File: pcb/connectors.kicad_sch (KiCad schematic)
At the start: 5 parts, among them CN1 STDC14, CN2 SM04B-SRSS-TB (LF)(SN), CN4 SM04B-SRSS-TB (LF)(SN), J1 Conn_01x12, J2 Conn_01x16

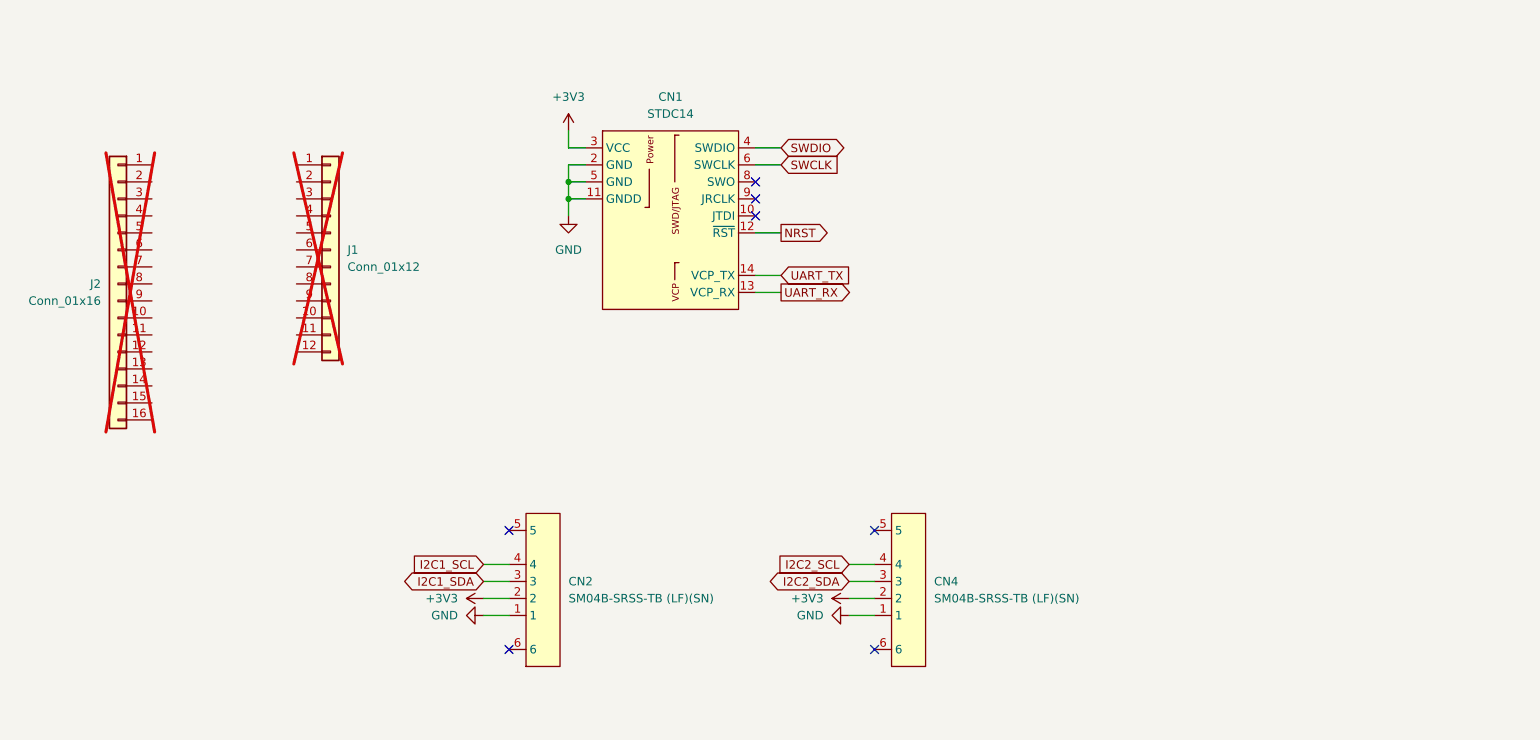
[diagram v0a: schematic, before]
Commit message: Lots of work on schematics
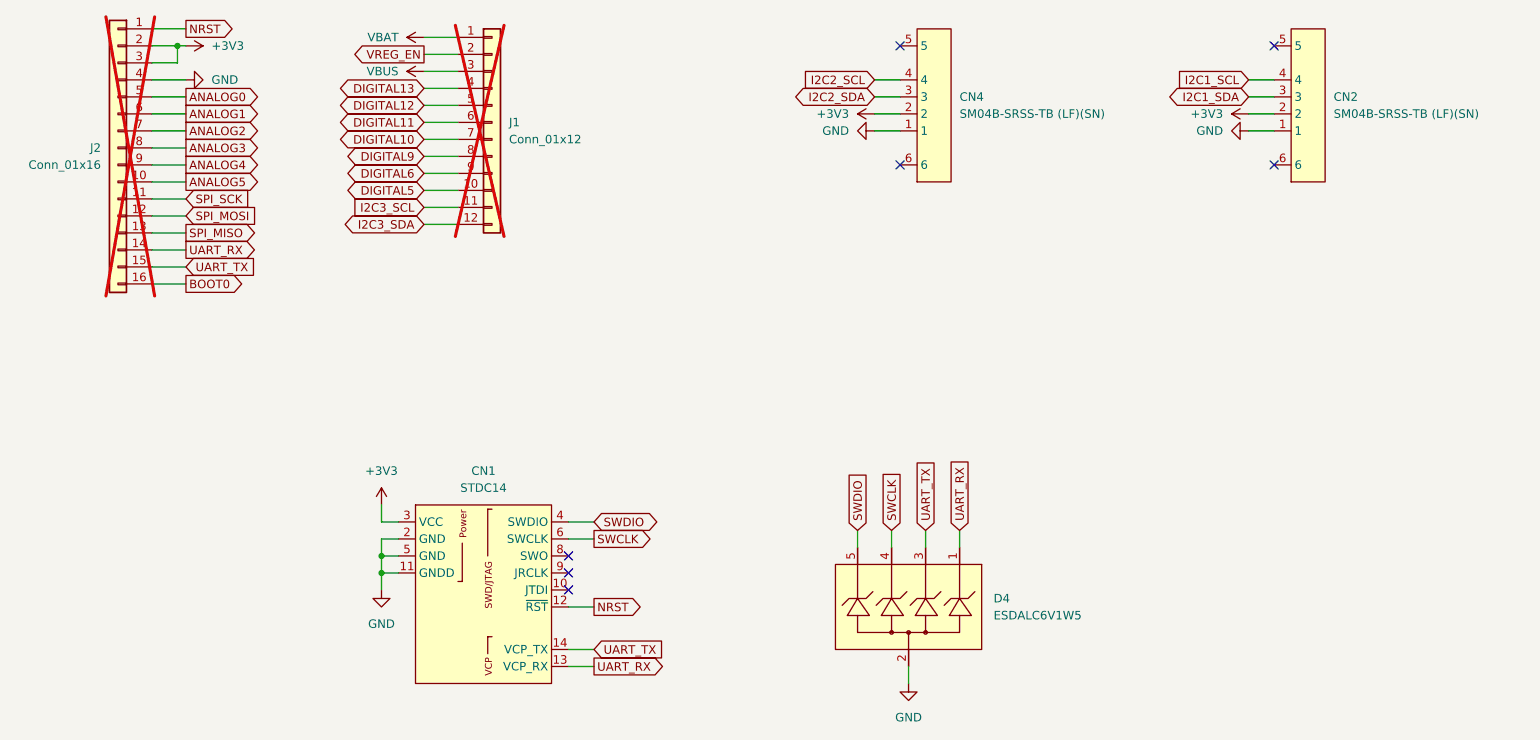
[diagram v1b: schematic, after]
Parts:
- added D4: ESDALC6V1W5, prop-devboard:SOT-323-5_L2.0-W1.3-LS2.1-BL, symbol prop-devboard:ESDALC6V1W5
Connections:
- net +3V3: now also J2.2 (Pin_2), J2.3 (Pin_3)
- net GND: now also J2.4 (Pin_4), D4.2
- net NRST: now also J2.1 (Pin_1)
- net SWCLK: now also D4.4
- net SWDIO: now also D4.5
- net UART_RX: now also J2.14 (Pin_14), D4.1
- net UART_TX: now also J2.15 (Pin_15), D4.3
- net ANALOG5: now reaches J2.10 (Pin_10)
- net SPI_SCK: now reaches J2.11 (Pin_11)
- net SPI_MOSI: now reaches J2.12 (Pin_12)
- net SPI_MISO: now reaches J2.13 (Pin_13)
- net BOOT0: now reaches J2.16 (Pin_16)
- net ANALOG0: now reaches J2.5 (Pin_5)
- net ANALOG1: now reaches J2.6 (Pin_6)
- net ANALOG2: now reaches J2.7 (Pin_7)
- net ANALOG3: now reaches J2.8 (Pin_8)
- net ANALOG4: now reaches J2.9 (Pin_9)
- net VBAT: now reaches J1.1 (Pin_1)
- net DIGITAL5: now reaches J1.10 (Pin_10)
- net I2C3_SCL: now reaches J1.11 (Pin_11)
- net I2C3_SDA: now reaches J1.12 (Pin_12)
- net VREG_EN: now reaches J1.2 (Pin_2)
- net VBUS: now reaches J1.3 (Pin_3)
- net DIGITAL13: now reaches J1.4 (Pin_4)
- net DIGITAL12: now reaches J1.5 (Pin_5)
- net DIGITAL11: now reaches J1.6 (Pin_6)
- net DIGITAL10: now reaches J1.7 (Pin_7)
- net DIGITAL9: now reaches J1.8 (Pin_8)
- net DIGITAL6: now reaches J1.9 (Pin_9)
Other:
- moved on the sheet: CN1, CN2, CN4, J1, J2
